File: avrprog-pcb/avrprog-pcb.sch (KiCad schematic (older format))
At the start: 28 parts, among them J1 Conn_01x04, J2 em_clk, U1 FT232RL, U2 ATmega8A-PU

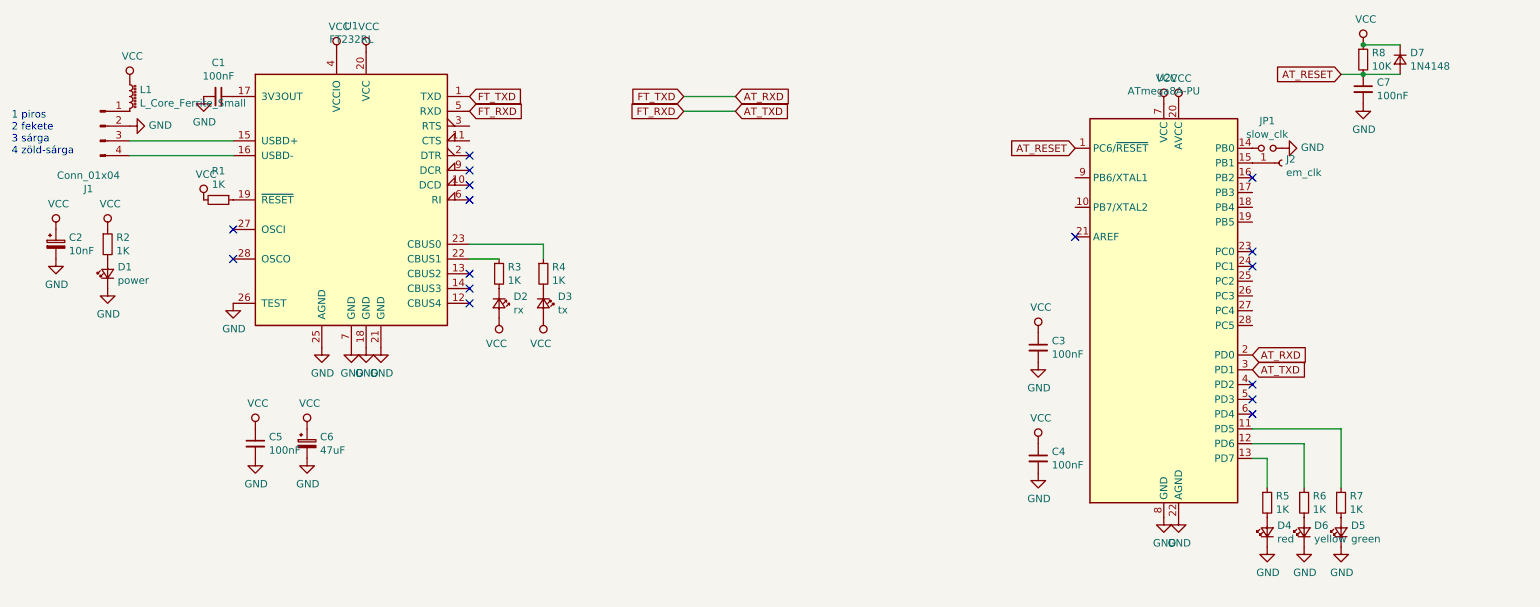
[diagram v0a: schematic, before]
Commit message: creating PCB
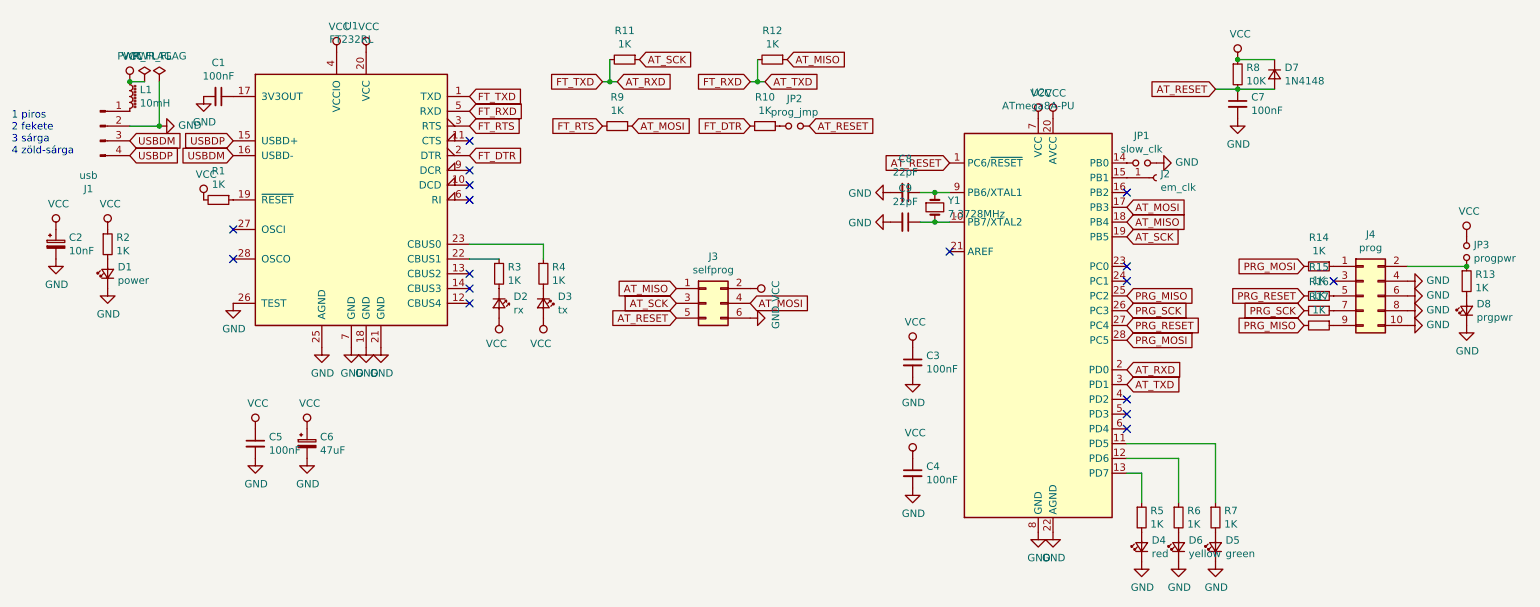
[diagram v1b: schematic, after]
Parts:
- added C8, C9: 22pF, Capacitor_THT:C_Disc_D5.0mm_W2.5mm_P2.50mm, symbol Device:C_Small
- added D8: prgpwr, LED_THT:LED_D3.0mm, symbol Device:LED_Small
- added J3: selfprog, Connector_PinHeader_2.54mm:PinHeader_2x03_P2.54mm_Vertical, symbol Connector_Generic:Conn_02x03_Odd_Even
- added J4: prog, Connector_PinHeader_2.54mm:PinHeader_2x05_P2.54mm_Vertical, symbol Connector_Generic:Conn_02x05_Odd_Even
- added JP2: prog_jmp, Connector_PinHeader_2.54mm:PinHeader_1x02_P2.54mm_Vertical, symbol Device:Jumper_NO_Small
- added JP3: progpwr, Connector_PinHeader_2.54mm:PinHeader_1x02_P2.54mm_Vertical, symbol Device:Jumper_NO_Small
- added R10, R11, R12, R13, R14, R15, R16, R17, R9: 1K, Resistor_THT:R_Axial_DIN0207_L6.3mm_D2.5mm_P10.16mm_Horizontal, symbol Device:R_Small
- added Y1: 7.3728MHz, Crystal:Crystal_HC49-U_Vertical, symbol Device:Crystal_Small
- C1, C2, C3, C4, C5, C7: footprint (none) -> Capacitor_THT:C_Disc_D5.0mm_W2.5mm_P2.50mm
- C6: footprint (none) -> Capacitor_THT:CP_Radial_D6.3mm_P2.50mm
- D1, D2, D3, D4, D5, D6: footprint (none) -> LED_THT:LED_D3.0mm
- D7: footprint (none) -> Diode_THT:D_DO-35_SOD27_P7.62mm_Horizontal
- J1: value Conn_01x04 -> usb
- L1: value L_Core_Ferrite_Small -> 10mH; footprint (none) -> Inductor_THT:L_Axial_L6.6mm_D2.7mm_P10.16mm_Horizontal_Vishay_IM-2
- R1, R2, R3, R4, R5, R6, R7, R8: footprint (none) -> Resistor_THT:R_Axial_DIN0207_L6.3mm_D2.5mm_P10.16mm_Horizontal
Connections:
- net AT_RESET: now also J3.5 (Pin_5), JP2.2
- net AT_RXD: now also R11.2
- net AT_TXD: now also R12.2
- net GND: now also C8.2, C9.2, D8.1 (K), J3.6 (Pin_6), J4.10 (Pin_10), J4.4 (Pin_4), J4.6 (Pin_6), J4.8 (Pin_8)
- net VCC: now also J3.2 (Pin_2), JP3.1
- net USBDM: now reaches J1.3 (Pin_3)
- net USBDM: now also U1.16 (USBD-); no longer U1.15 (USBD+)
- net USBDP: now reaches J1.4 (Pin_4)
- net USBDP: now also U1.15 (USBD+); no longer U1.16 (USBD-)
- net FT_DTR: now reaches U1.2 (DTR)
- net FT_DTR: now also R10.2
- net FT_RTS: now reaches U1.3 (RTS)
- net FT_RTS: now also R9.2
- net at U2.10 (PB7/XTAL2): now also C9.1, Y1.2
- net AT_MOSI: now reaches U2.17 (PB3)
- net AT_MOSI: now also J3.4 (Pin_4), R9.1
- net AT_MISO: now reaches U2.18 (PB4)
- net AT_MISO: now also J3.1 (Pin_1), R12.1
- net AT_SCK: now reaches U2.19 (PB5)
- net AT_SCK: now also J3.3 (Pin_3), R11.1
- net PRG_MISO: now reaches U2.25 (PC2)
- net PRG_MISO: now also R17.2
- net PRG_SCK: now reaches U2.26 (PC3)
- net PRG_SCK: now also R16.2
- net PRG_RESET: now reaches U2.27 (PC4)
- net PRG_RESET: now also R15.2
- net PRG_MOSI: now reaches U2.28 (PC5)
- net PRG_MOSI: now also R14.2
- net at U2.9 (PB6/XTAL1): now also C8.1, Y1.1
- new net: JP2.1, R10.1
- new net: J4.1 (Pin_1), R14.1
- new net: J4.2 (Pin_2), JP3.2, R13.1
- new net: J4.5 (Pin_5), R15.1
- new net: J4.7 (Pin_7), R16.1
- new net: J4.9 (Pin_9), R17.1
- new net: D8.2 (A), R13.2
- no-connect marks 16 -> 17
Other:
- moved on the sheet: C3, C4, C7, D4, D5, D6, D7, J2, JP1, R5, R6, R7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

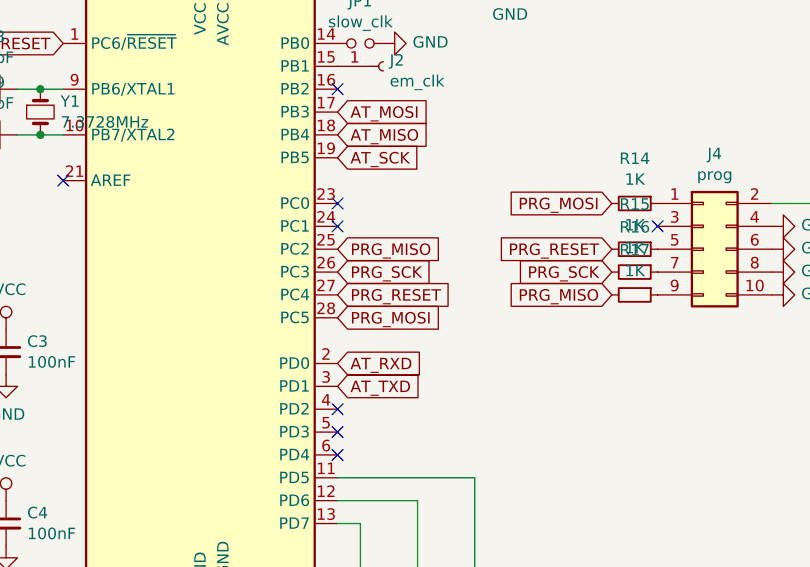
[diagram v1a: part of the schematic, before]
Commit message: designing PCB
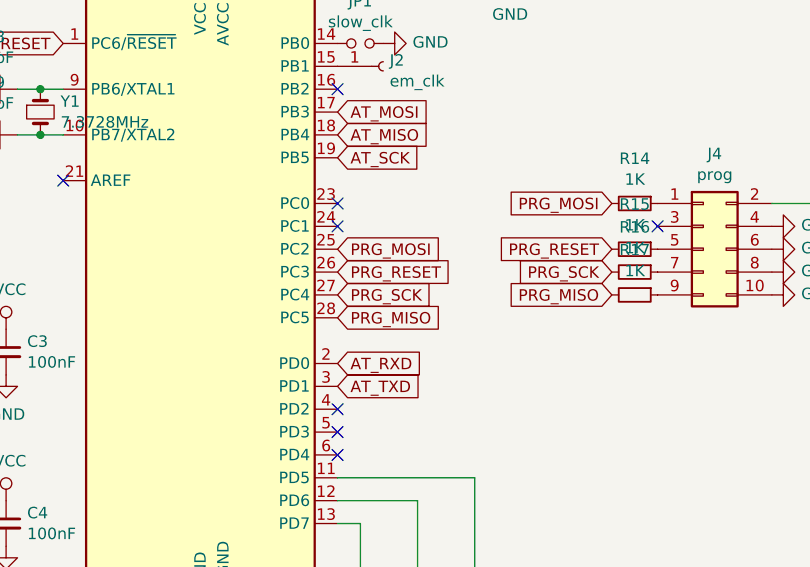
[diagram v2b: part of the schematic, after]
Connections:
- net PRG_MISO: now also U2.28 (PC5); no longer U2.25 (PC2)
- net PRG_MOSI: now also U2.25 (PC2); no longer U2.28 (PC5)
- net PRG_RESET: now also U2.26 (PC3); no longer U2.27 (PC4)
- net PRG_SCK: now also U2.27 (PC4); no longer U2.26 (PC3)
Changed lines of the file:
@@
 Text GLabel 9400 3450 0    50   Input ~ 0
 PRG_MOSI
-Text GLabel 8200 3950 2    50   Input ~ 0
+Text GLabel 8200 3650 2    50   Input ~ 0
 PRG_MOSI
-Text GLabel 8200 3850 2    50   Input ~ 0
+Text GLabel 8200 3750 2    50   Input ~ 0
 PRG_RESET
 Text GLabel 9400 3650 0    50   Input ~ 0
 PRG_RESET
-Text GLabel 8200 3750 2    50   Input ~ 0
+Text GLabel 8200 3850 2    50   Input ~ 0
 PRG_SCK
 Text GLabel 9400 3750 0    50   Input ~ 0
 PRG_SCK
-Text GLabel 8200 3650 2    50   Input ~ 0
+Text GLabel 8200 3950 2    50   Input ~ 0
 PRG_MISO
 Text GLabel 9400 3850 0    50   Input ~ 0
